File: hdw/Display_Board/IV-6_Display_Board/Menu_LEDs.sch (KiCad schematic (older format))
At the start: 1 part

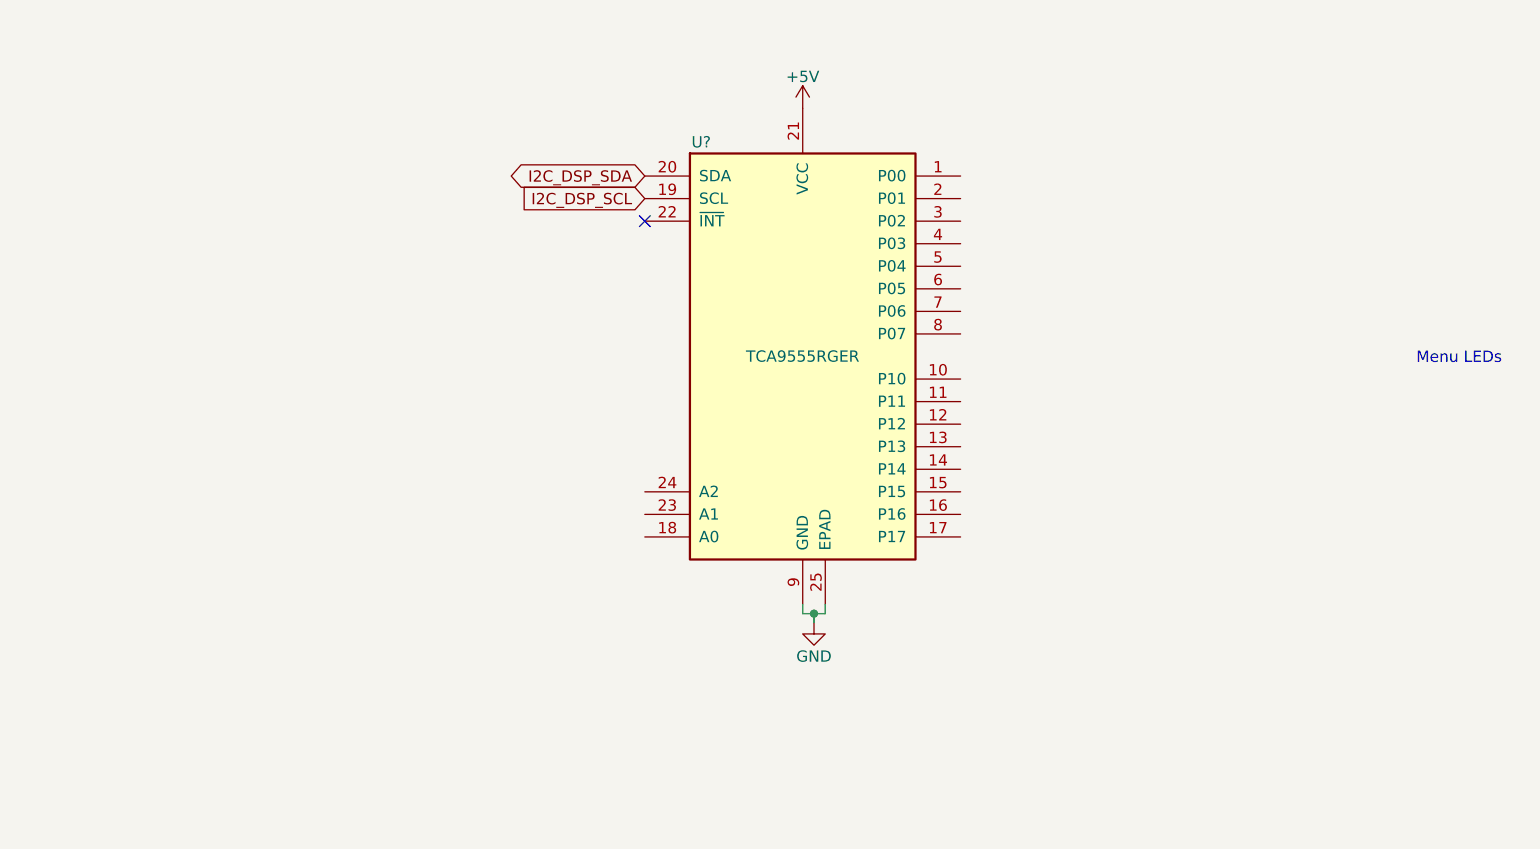
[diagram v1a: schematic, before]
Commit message: Display board tweaks, added buzzer, other stuff
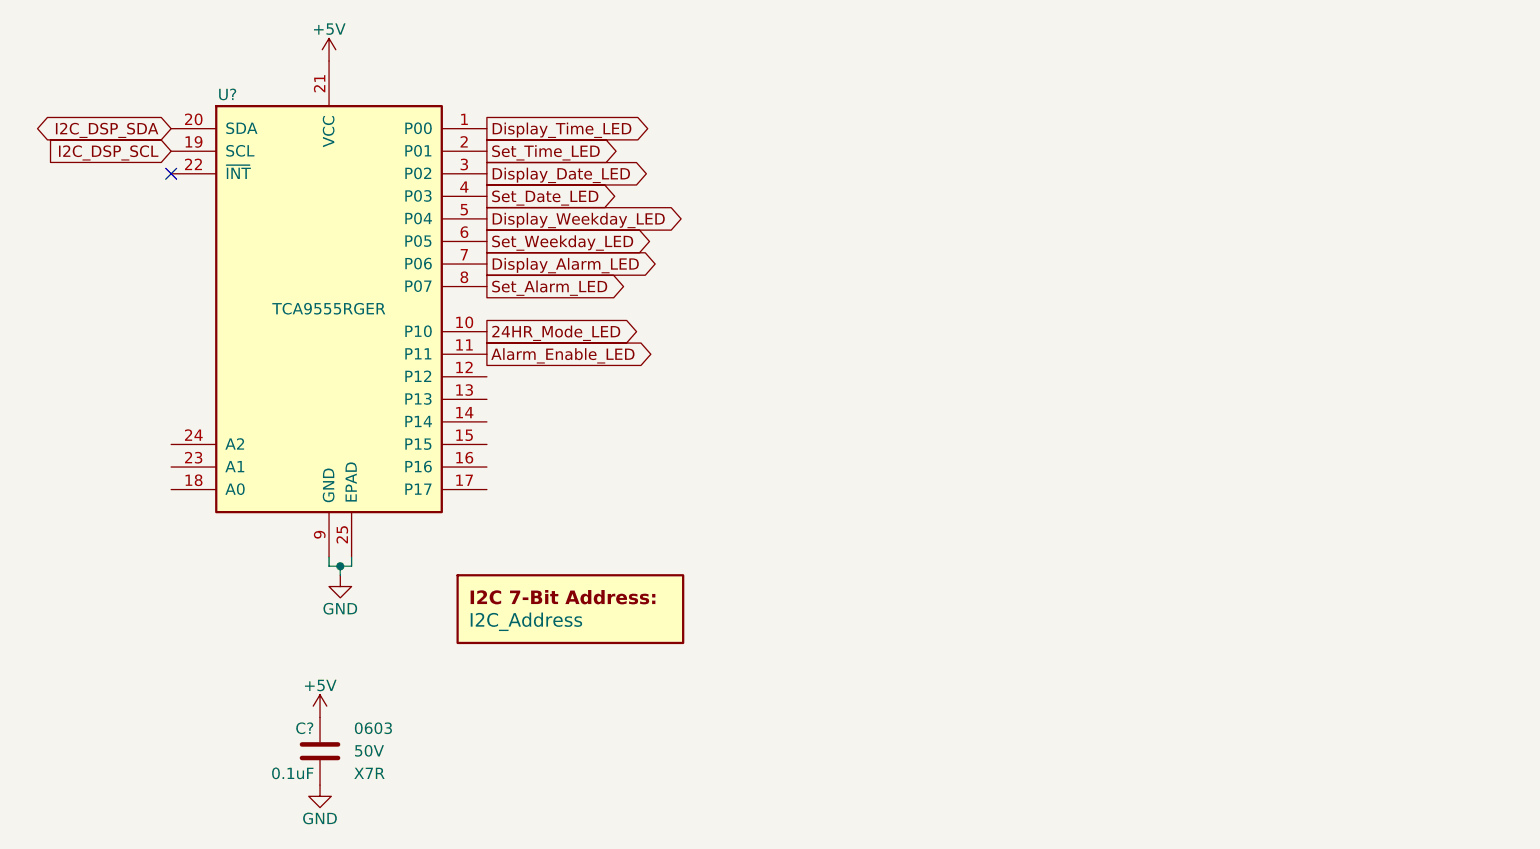
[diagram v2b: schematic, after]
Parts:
- added C?: 0.1uF, Capacitors_SMD:C_0603, symbol Custom_Library:C_Custom
- added DOC?: I2C_Address, symbol Custom_Library:I2C_Address
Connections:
- net +5V: now also C?.1
- net GND: now also C?.2
- net Display_Time_LED: now reaches U?.1 (P00)
- net 24HR_Mode_LED: now reaches U?.10 (P10)
- net Alarm_Enable_LED: now reaches U?.11 (P11)
- net Set_Time_LED: now reaches U?.2 (P01)
- net Display_Date_LED: now reaches U?.3 (P02)
- net Set_Date_LED: now reaches U?.4 (P03)
- net Display_Weekday_LED: now reaches U?.5 (P04)
- net Set_Weekday_LED: now reaches U?.6 (P05)
- net Display_Alarm_LED: now reaches U?.7 (P06)
- net Set_Alarm_LED: now reaches U?.8 (P07)
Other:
- note removed: "Menu LEDs"
- moved on the sheet: U?
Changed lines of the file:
@@
 $Descr A 11000 8500
 encoding utf-8
-Sheet 5 9
+Sheet 5 12
 Title ""
 Date ""
@@
 L Interface_Expansion:TCA9555RGER U?
 U 1 1 5E0AA272
-P 5060 3310
-F 0 "U?" H 4610 4260 50  0000 C CNN
-F 1 "TCA9555RGER" H 5060 3310 50  0000 C CNN
-F 2 "Package_DFN_QFN:QFN-24-1EP_4x4mm_P0.5mm_EP2.6x2.6mm" H 6260 2310 50  0001 C CNN
-F 3 "http://www.ti.com/lit/ds/symlink/tca9555.pdf" H 4560 4210 50  0001 C CNN
-	1    5060 3310
+P 2960 3100
+F 0 "U?" H 2510 4050 50  0000 C CNN
+F 1 "TCA9555RGER" H 2960 3100 50  0000 C CNN
+F 2 "Package_DFN_QFN:QFN-24-1EP_4x4mm_P0.5mm_EP2.6x2.6mm" H 4160 2100 50  0001 C CNN
+F 3 "http://www.ti.com/lit/ds/symlink/tca9555.pdf" H 2460 4000 50  0001 C CNN
+	1    2960 3100
 	1    0    0    -1
 $EndComp
@@
 L power:+5V #PWR?
 U 1 1 5E0AB497
-P 5060 2210
-F 0 "#PWR?" H 5060 2060 50  0001 C CNN
-F 1 "+5V" H 5060 2350 50  0000 C CNN
-F 2 "" H 5060 2210 50  0001 C CNN
-F 3 "" H 5060 2210 50  0001 C CNN
-	1    5060 2210
+P 2960 2000
+F 0 "#PWR?" H 2960 1850 50  0001 C CNN
+F 1 "+5V" H 2960 2140 50  0000 C CNN
+F 2 "" H 2960 2000 50  0001 C CNN
+F 3 "" H 2960 2000 50  0001 C CNN
+	1    2960 2000
 	1    0    0    -1
 $EndComp
@@
 L power:GND #PWR?
 U 1 1 5E0AB88F
-P 5110 4490
-F 0 "#PWR?" H 5110 4240 50  0001 C CNN
-F 1 "GND" H 5110 4340 50  0000 C CNN
-F 2 "" H 5110 4490 50  0001 C CNN
-F 3 "" H 5110 4490 50  0001 C CNN
-	1    5110 4490
+P 3010 4280
+F 0 "#PWR?" H 3010 4030 50  0001 C CNN
+F 1 "GND" H 3010 4130 50  0000 C CNN
+F 2 "" H 3010 4280 50  0001 C CNN
+F 3 "" H 3010 4280 50  0001 C CNN
+	1    3010 4280
 	1    0    0    -1
 $EndComp
 Wire Wire Line
-	5110 4490 5110 4450
+	3010 4280 3010 4240
 Wire Wire Line
-	5110 4450 5060 4450
+	3010 4240 2960 4240
 Wire Wire Line
-	5060 4450 5060 4410
+	2960 4240 2960 4200
 Wire Wire Line
-	5110 4450 5160 4450
+	3010 4240 3060 4240
 Wire Wire Line
-	5160 4450 5160 4410
-Connection ~ 5110 4450
-NoConn ~ 4360 2710
-Text GLabel 4360 2510 0    50   BiDi ~ 0
+	3060 4240 3060 4200
+Connection ~ 3010 4240
+NoConn ~ 2260 2500
+Text GLabel 2260 2300 0    50   BiDi ~ 0
 I2C_DSP_SDA
-Text GLabel 4360 2610 0    50   Input ~ 0
+Text GLabel 2260 2400 0    50   Input ~ 0
 I2C_DSP_SCL
-Text Notes 7780 3350 0    50   ~ 0
-Menu LEDs
+Text GLabel 3660 3200 2    50   Output ~ 0
+24HR_Mode_LED
+Text GLabel 3660 2300 2    50   Output ~ 0
+Display_Time_LED
+Text GLabel 3660 2500 2    50   Output ~ 0
+Display_Date_LED
+Text GLabel 3660 2900 2    50   Output ~ 0
+Display_Alarm_LED
+Text GLabel 3660 2400 2    50   Output ~ 0
+Set_Time_LED
+Text GLabel 3660 2600 2    50   Output ~ 0
+Set_Date_LED
+Text GLabel 3660 3000 2    50   Output ~ 0
+Set_Alarm_LED
+Text GLabel 3660 2700 2    50   Output ~ 0
+Display_Weekday_LED
+Text GLabel 3660 2800 2    50   Output ~ 0
+Set_Weekday_LED
+$Comp
+L Custom_Library:I2C_Address DOC?
+U 1 1 5E3D77B3
+P 4030 4480
+F 0 "DOC?" H 4030 4730 60  0001 C CNN
+F 1 "I2C_Address" H 3580 4480 60  0000 L CNN
+F 2 "" H 4030 4830 60  0001 C CNN
+F 3 "" H 4030 4830 60  0001 C CNN
+	1    4030 4480
+	1    0    0    -1
+$EndComp
+Text GLabel 3660 3300 2    50   Output ~ 0
+Alarm_Enable_LED
+$Comp
+L Custom_Library:C_Custom C?
+U 1 1 5E25E93E
+P 2920 5060
+AR Path="/5C1D5CD8/5E25E93E" Ref="C?"  Part="1"
+AR Path="/5C1D5CCA/5E25E93E" Ref="C?"  Part="1"
+AR Path="/5C26E09A/5E25E93E" Ref="C?"  Part="1"
+AR Path="/5D739492/5E25E93E" Ref="C?"  Part="1"
+AR Path="/5E28CFDF/5E25E93E" Ref="C?"  Part="1"
+AR Path="/5E36CE18/5E25E93E" Ref="C?"  Part="1"
+AR Path="/5E3C80C8/5E25E93E" Ref="C?"  Part="1"
+AR Path="/5E3C97B4/5E25E93E" Ref="C?"  Part="1"
+AR Path="/5E0A7959/5E25E93E" Ref="C?"  Part="1"
+F 0 "C?" H 2945 5160 50  0000 L CNN
+F 1 "0.1uF" H 2945 4960 50  0000 L CNN
+F 2 "Capacitors_SMD:C_0603" H 2958 4910 50  0001 C CNN
+F 3 "" H 2945 5160 50  0001 C CNN
+F 4 "311-1344-1-ND" H 3345 5560 60  0001 C CNN "Digi-Key PN"
+F 5 "0603" H 2770 5160 50  0000 R CNN "display_footprint"
+F 6 "50V" H 2770 5060 50  0000 R CNN "Voltage"
+F 7 "X7R" H 2770 4960 50  0000 R CNN "Dielectric"
+	1    2920 5060
+	-1   0    0    -1
+$EndComp
+$Comp
+L power:GND #PWR?
+U 1 1 5E25E944
+P 2920 5210
+AR Path="/5E28CFDF/5E25E944" Ref="#PWR?"  Part="1"
+AR Path="/5E36CE18/5E25E944" Ref="#PWR?"  Part="1"
+AR Path="/5E3C80C8/5E25E944" Ref="#PWR?"  Part="1"
+AR Path="/5E3C97B4/5E25E944" Ref="#PWR?"  Part="1"
+AR Path="/5E0A7959/5E25E944" Ref="#PWR?"  Part="1"
+F 0 "#PWR?" H 2920 4960 50  0001 C CNN
+F 1 "GND" H 2920 5060 50  0000 C CNN
+F 2 "" H 2920 5210 50  0001 C CNN
+F 3 "" H 2920 5210 50  0001 C CNN
+	1    2920 5210
+	1    0    0    -1
+$EndComp
+$Comp
+L power:+5V #PWR?
+U 1 1 5E25E974
+P 2920 4910
+F 0 "#PWR?" H 2920 4760 50  0001 C CNN
+F 1 "+5V" H 2920 5050 50  0000 C CNN
+F 2 "" H 2920 4910 50  0001 C CNN
+F 3 "" H 2920 4910 50  0001 C CNN
+	1    2920 4910
+	1    0    0    -1
+$EndComp
 $EndSCHEMATC
